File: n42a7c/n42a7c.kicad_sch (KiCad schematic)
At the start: 111 parts, among them J1 Conn_01x02, J2 Conn_01x03, SW1 CPG151101S11-16, SW10 CPG151101S11-16, SW11 CPG151101S11-16, SW12 CPG151101S11-16, SW13 CPG151101S11-16, SW14 CPG151101S11-16, SW15 CPG151101S11-16, SW16 CPG151101S11-16, SW17 CPG151101S11-16, SW18 CPG151101S11-16, SW19 CPG151101S11-16, SW2 CPG151101S11-16, SW20 CPG151101S11-16, SW21 CPG151101S11-16, SW22 CPG151101S11-16, SW23 CPG151101S11-16, SW24 CPG151101S11-16, SW25 CPG151101S11-16, SW26 CPG151101S11-16, SW27 CPG151101S11-16, SW28 CPG151101S11-16, SW29 CPG151101S11-16, SW3 CPG151101S11-16, SW30 CPG151101S11-16, SW31 CPG151101S11-16, SW32 CPG151101S11-16, SW33 CPG151101S11-16, SW34 CPG151101S11-16, SW35 CPG151101S11-16, SW36 CPG151101S11-16, SW37 CPG151101S11-16, SW38 CPG151101S11-16, SW39 CPG151101S11-16, SW4 CPG151101S11-16, SW40 CPG151101S11-16, SW41 CPG151101S11-16, SW42 CPG151101S11-16, SW5 CPG151101S11-16, SW6 CPG151101S11-16, SW7 CPG151101S11-16, SW8 CPG151101S11-16, SW9 CPG151101S11-16, U1 XIAO-nRF52840-SMD

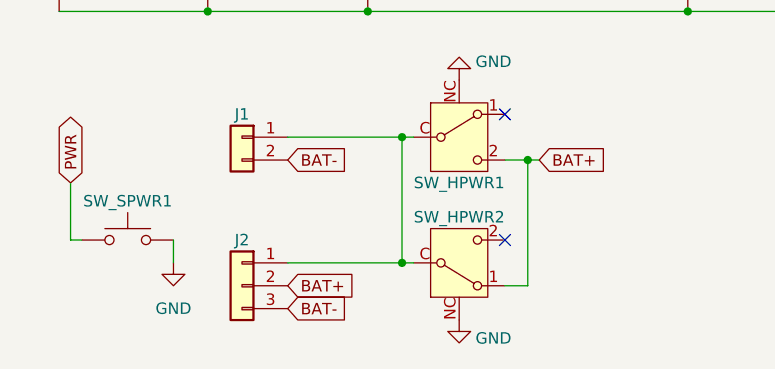
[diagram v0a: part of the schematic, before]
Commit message: revise switch
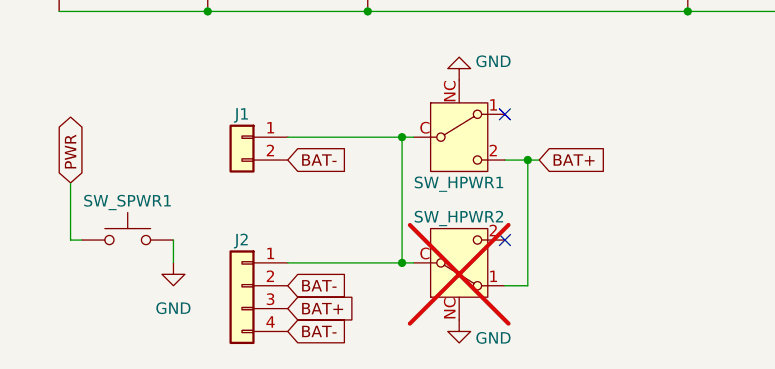
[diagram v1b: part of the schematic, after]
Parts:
- J2: footprint Connector_PinHeader_2.00mm:PinHeader_1x03_P2.00mm_Vertical -> Connector_PinHeader_2.00mm:PinHeader_1x04_P2.00mm_Vertical; symbol Connector_Generic:Conn_01x03 -> Connector_Generic:Conn_01x04
- SW_HPWR1: value SSAJ110100 -> SK-12D11; footprint cscslib:SSAJ110100 -> cscslib:SK-12D11
- SW_HPWR2: footprint cscslib:SSAJ110100 -> cscslib:SK-12D11; now not fitted; now left out of the parts list
- SW_SPWR1: value SW_SPWR -> THAU13-AB-R
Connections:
- net BAT+: now also J2.3 (Pin_3); no longer J2.2 (Pin_2)
- net BAT-: now also J2.2 (Pin_2), J2.4 (Pin_4); no longer J2.3 (Pin_3)
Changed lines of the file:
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@@
 	(global_label "BAT-"
 		(shape input)
-		(at 43.18 189.23 0)
+		(at 43.18 191.77 0)
 		(effects
 			(font
@@
 		)
 		(property "Intersheetrefs" "${INTERSHEET_REFS}"
-			(at 43.18 189.23 90)
+			(at 43.18 191.77 90)
 			(effects
 				(font
@@
 		)
 	)
+	(global_label "BAT-"
+		(shape input)
+		(at 43.18 186.69 0)
+		(effects
+			(font
+				(size 1.27 1.27)
+			)
+			(justify left)
+		)
+		(property "Intersheetrefs" "${INTERSHEET_REFS}"
+			(at 43.18 186.69 90)
+			(effects
+				(font
+					(size 1.27 1.27)
+				)
+				(hide yes)
+			)
+		)
+	)
 	(global_label "IO 3"
 		(shape bidirectional)
@@
 	(global_label "BAT+"
 		(shape input)
-		(at 43.18 186.69 0)
+		(at 43.18 189.23 0)
 		(effects
 			(font
@@
 		)
 		(property "Intersheetrefs" "${INTERSHEET_REFS}"
-			(at 43.18 186.69 90)
+			(at 43.18 189.23 90)
 			(effects
 				(font
@@
 			)
 		)
-		(property "Value" "SW_SPWR"
+		(property "Value" "THAU13-AB-R"
 			(at 25.4 183.134 0)
 			(effects
@@
 	)
 	(symbol
-		(lib_id "Connector_Generic:Conn_01x03")
+		(lib_id "Connector_Generic:Conn_01x04")
 		(at 38.1 186.69 0)
 		(mirror y)
@@
 			)
 		)
-		(property "Footprint" "Connector_PinHeader_2.00mm:PinHeader_1x03_P2.00mm_Vertical"
+		(property "Footprint" "Connector_PinHeader_2.00mm:PinHeader_1x04_P2.00mm_Vertical"
 			(at 38.1 186.69 0)
 			(effects
@@
 			)
 		)
-		(property "Description" "Generic connector, single row, 01x03, script generated (kicad-library-utils/schlib/autogen/connector/)"
+		(property "Description" "Generic connector, single row, 01x04, script generated (kicad-library-utils/schlib/autogen/connector/)"
 			(at 38.1 186.69 0)
 			(effects
@@
 		(pin "3"
 		)
+		(pin "4"
+		)
 		(instances
 			(project ""
@@
 		(unit 1)
 		(exclude_from_sim no)
-		(in_bom yes)
-		(on_board yes)
-		(dnp no)
+		(in_bom no)
+		(on_board no)
+		(dnp yes)
 		(property "Reference" "SW_HPWR2"
 			(at 62.23 179.07 0)
@@
 			)
 		)
-		(property "Footprint" "cscslib:SSAJ110100"
+		(property "Footprint" "cscslib:SK-12D11"
 			(at 62.23 184.15 0)
 			(effects
@@
 			)
 		)
-		(property "Value" "SSAJ110100"
+		(property "Value" "SK-12D11"
 			(at 62.23 175.26 0)
 			(effects
@@
 			)
 		)
-		(property "Footprint" "cscslib:SSAJ110100"
+		(property "Footprint" "cscslib:SK-12D11"
 			(at 62.23 170.18 0)
 			(effects
